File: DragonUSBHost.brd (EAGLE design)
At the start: 49.5 x 59.7 mm, 30 parts, among them IC1 MAX3421EEHJ, J1 Dragino, J2 MICROSD, J3 Sensors, J4 Serial, J5 XBee, P1 USB_, Q1 12 MHz

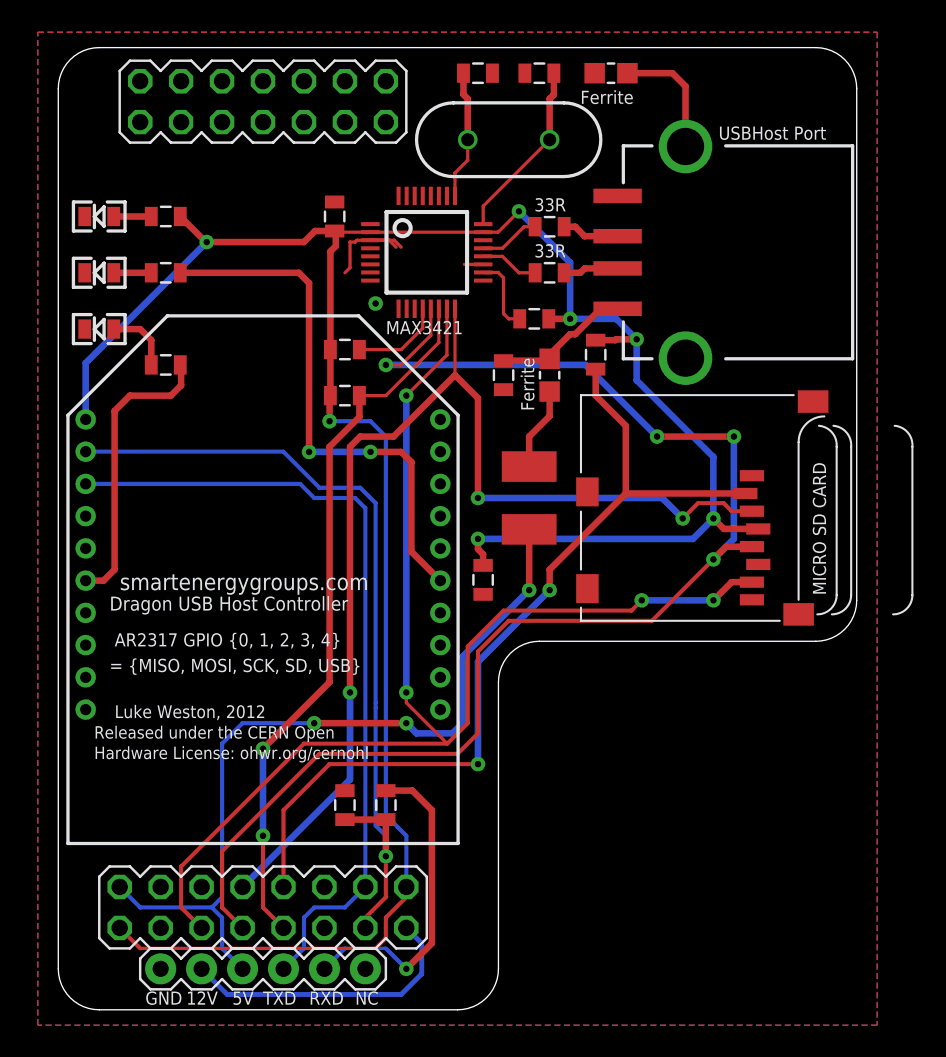
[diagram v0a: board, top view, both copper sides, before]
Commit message: foo
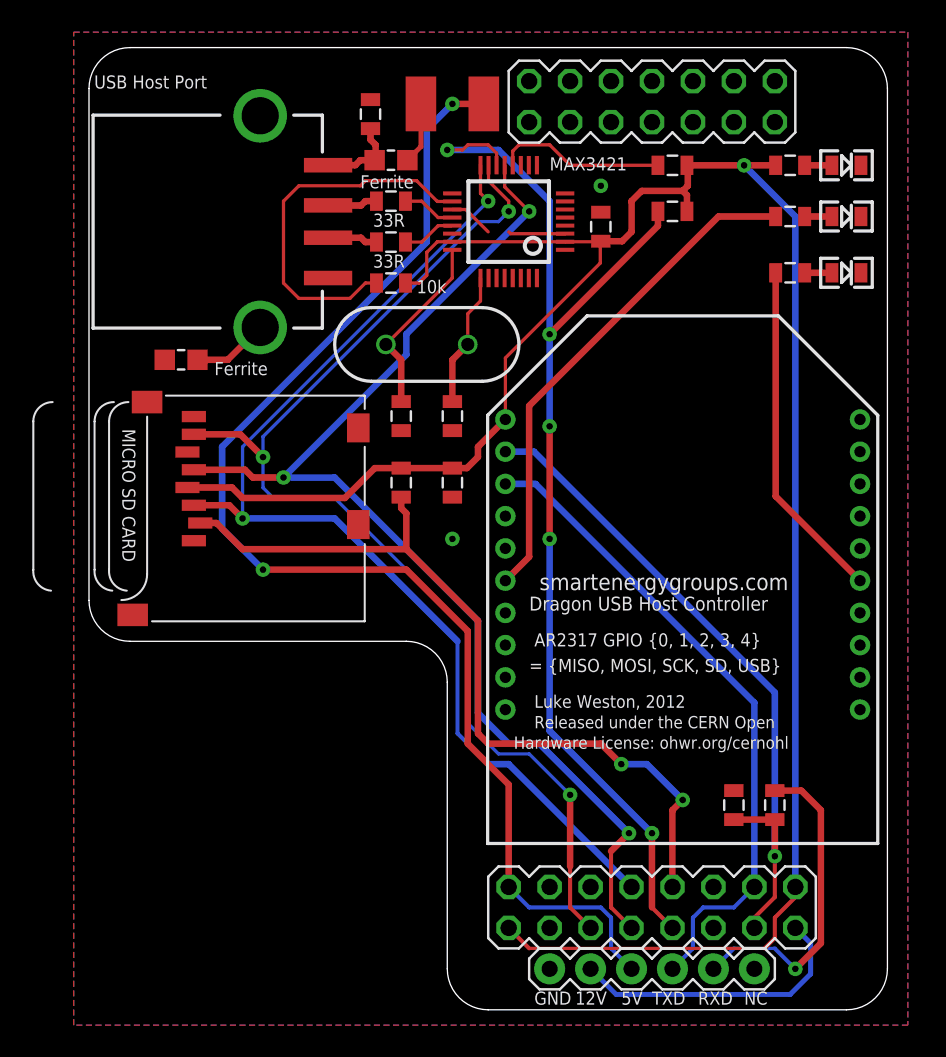
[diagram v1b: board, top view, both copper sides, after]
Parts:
- moved LED1 46.9 mm to (48.9, 49.2), turned to 0 degrees
- moved LED3 46.5 mm to (48.9, 52.4), turned to 0 degrees
- moved LED2 46.4 mm to (48.9, 45.7), turned to 0 degrees
- moved R4 39.8 mm to (45.4, 49.2), turned to 180 degrees
- moved R11 38.9 mm to (45.4, 52.4), turned to 180 degrees
- moved R5 38.7 mm to (45.4, 45.7), turned to 180 degrees
- moved P1 32.4 mm to (9.53, 48.9), turned to 0 degrees
- moved L2 32.1 mm to (7.62, 40.3)
- moved J5 26.0 mm to (38.7, 27.6)
- moved F1 24.9 mm to (24.4, 56.2), turned to 0 degrees
- moved R2 24.1 mm to (44.5, 12.7)
- moved J1 24.1 mm to (36.8, 6.35)
- moved J3 24.1 mm to (36.8, 56.3)
- moved J4 24.1 mm to (36.8, 2.54)
- moved R3 24.1 mm to (41.9, 12.7)
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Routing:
- net +5V: track 51.0 -> 79.9 mm, vias 3 -> 2
- net !USB_CS: track 44.4 -> 70.5 mm, vias 2 -> 5
- net +3V3: track 151.7 -> 133.1 mm, vias 7 -> 1
- net !INTERRUPT: track 4.76 -> 23.2 mm
- net N$13: track 18.0 -> 31.6 mm
- net SCK: track 85.7 -> 72.9 mm, vias 4 -> 3
- net N$9: track 33.4 -> 21.3 mm, vias 2 -> 0
- net TXD: track 49.8 -> 40.8 mm
- net RXD: track 51.3 -> 42.8 mm
- net MISO: track 78.9 -> 71.5 mm, vias 4 -> 3
- net !RESET: track 5.68 -> 10.6 mm
- net !SDCARD_CS: track 54.5 -> 50.2 mm
- net N$4: track 8.62 -> 5.13 mm
- net N$2: track 7.68 -> 4.72 mm
- net N$12: track 4.15 -> 1.69 mm
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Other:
- outline, holes or cut-outs redrawn
- board text added: "10k"
- board text added: "USB Host Port"
- board text removed: "USBHost Port"
